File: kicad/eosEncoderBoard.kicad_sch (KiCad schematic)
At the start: 0 parts

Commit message: schematic half done
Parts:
- added DP1: Display1, Connector_PinSocket_2.54mm:PinSocket_1x04_P2.54mm_Vertical, symbol Connector_Generic:Conn_01x04
- added DP2: Display2, Connector_PinSocket_2.54mm:PinSocket_1x04_P2.54mm_Vertical, symbol Connector_Generic:Conn_01x04
- added DP3: Display3, Connector_PinSocket_2.54mm:PinSocket_1x04_P2.54mm_Vertical, symbol Connector_Generic:Conn_01x04
- added DP4: Display4, Connector_PinSocket_2.54mm:PinSocket_1x04_P2.54mm_Vertical, symbol Connector_Generic:Conn_01x04
- added R1, R10, R11, R12, R13, R14, R15, R16, R17, R18, R19, R2, R3, R4, R5, R6, R7, R8, R9: 10k, symbol Device:R_Small
- added SW1, SW2, SW3, SW4: RotaryEncoder, Rotary_Encoder:RotaryEncoder_Alps_EC11E-Switch_Vertical_H20mm_MountingHoles, symbol Device:RotaryEncoder_Switch_MP
- added U1: Teensy3.2, Teensy:Teensy30_31_32_LC, symbol Teensy:Teensy3.2
- added U2: PCA9548APW, Package_SO:TSSOP-24_4.4x7.8mm_P0.65mm, symbol Interface_Expansion:PCA9548APW
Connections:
- new net +3.3V: DP1.3 (Pin_3), DP2.3 (Pin_3), DP3.3 (Pin_3), DP4.3 (Pin_3), R1.1, R10.1, R11.1, R12.1, R13.2, R14.2, R15.2, R16.2, R17.2, R18.2, R19.2, R2.1, R3.1, R4.1, R5.1, R6.1, R7.1, R8.1, R9.1, U2.24 (VCC)
- new net A1: R2.2, SW1.A
- new net A2: R4.2, SW2.A
- new net A3: R7.2, SW3.A
- new net A4: R8.2, SW4.A
- new net B1: R1.2, SW1.B
- new net B2: R3.2, SW2.B
- new net B3: R5.2, SW3.B
- new net B4: R6.2, SW4.B
- new net GND: DP1.4 (Pin_4), DP2.4 (Pin_4), DP3.4 (Pin_4), DP4.4 (Pin_4), SW1.C, SW1.S2, SW2.C, SW2.S2, SW3.C, SW3.S2, SW4.C, SW4.S2, U2.1 (A0), U2.12 (GND), U2.2 (A1), U2.21 (A2)
- new net RST: R19.1, U2.3 (~{RESET})
- new net SCL: R17.1, U2.22 (SCL)
- new net SCL1: DP1.2 (Pin_2), R9.2, U2.5 (SC0)
- new net SCL2: DP2.2 (Pin_2), R11.2, U2.7 (SC1)
- new net SCL3: DP3.2 (Pin_2), R13.1, U2.9 (SC2)
- new net SCL4: DP4.2 (Pin_2), R15.1, U2.11 (SC3)
- new net SDA: R18.1, U2.23 (SDA)
- new net SDA1: DP1.1 (Pin_1), R10.2, U2.4 (SD0)
- new net SDA2: DP2.1 (Pin_1), R12.2, U2.6 (SD1)
- new net SDA3: DP3.1 (Pin_1), R14.1, U2.8 (SD2)
- new net SDA4: DP4.1 (Pin_1), R16.1, U2.10 (SD3)
- new net SW1: SW1.S1
- new net SW2: SW2.S1
- new net SW3: SW3.S1
- new net SW4: SW4.S1
- no-connect marks 0 -> 12
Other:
- note added: "Display Headers"
- note added: "Encoders"
- note added: "I2C Mux"

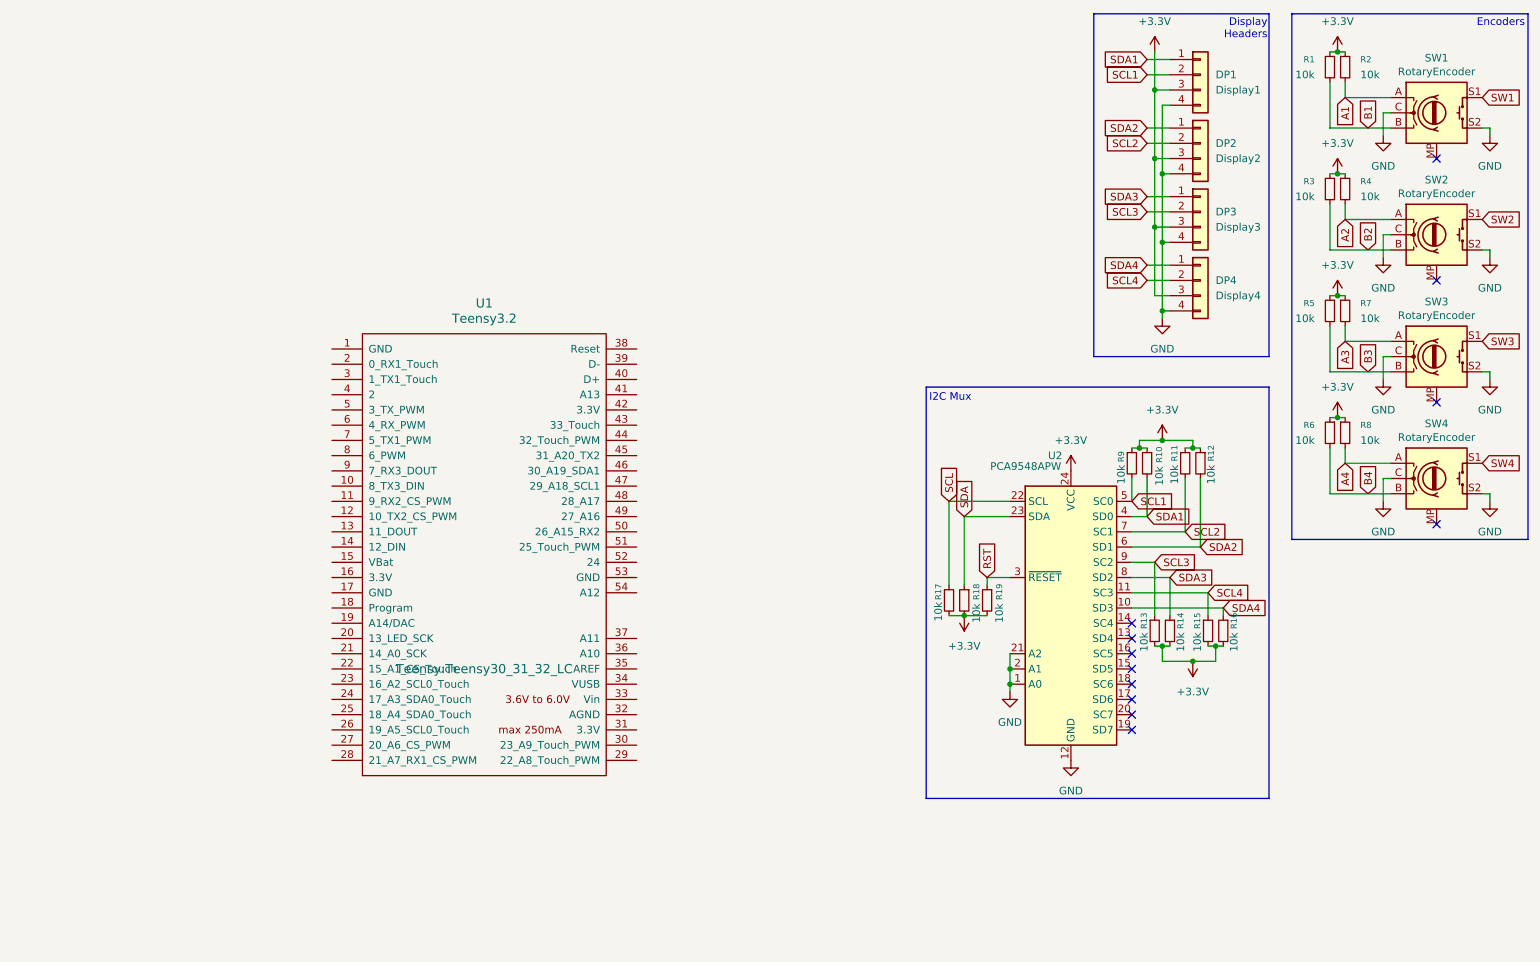
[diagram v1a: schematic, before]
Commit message: schematic basically done
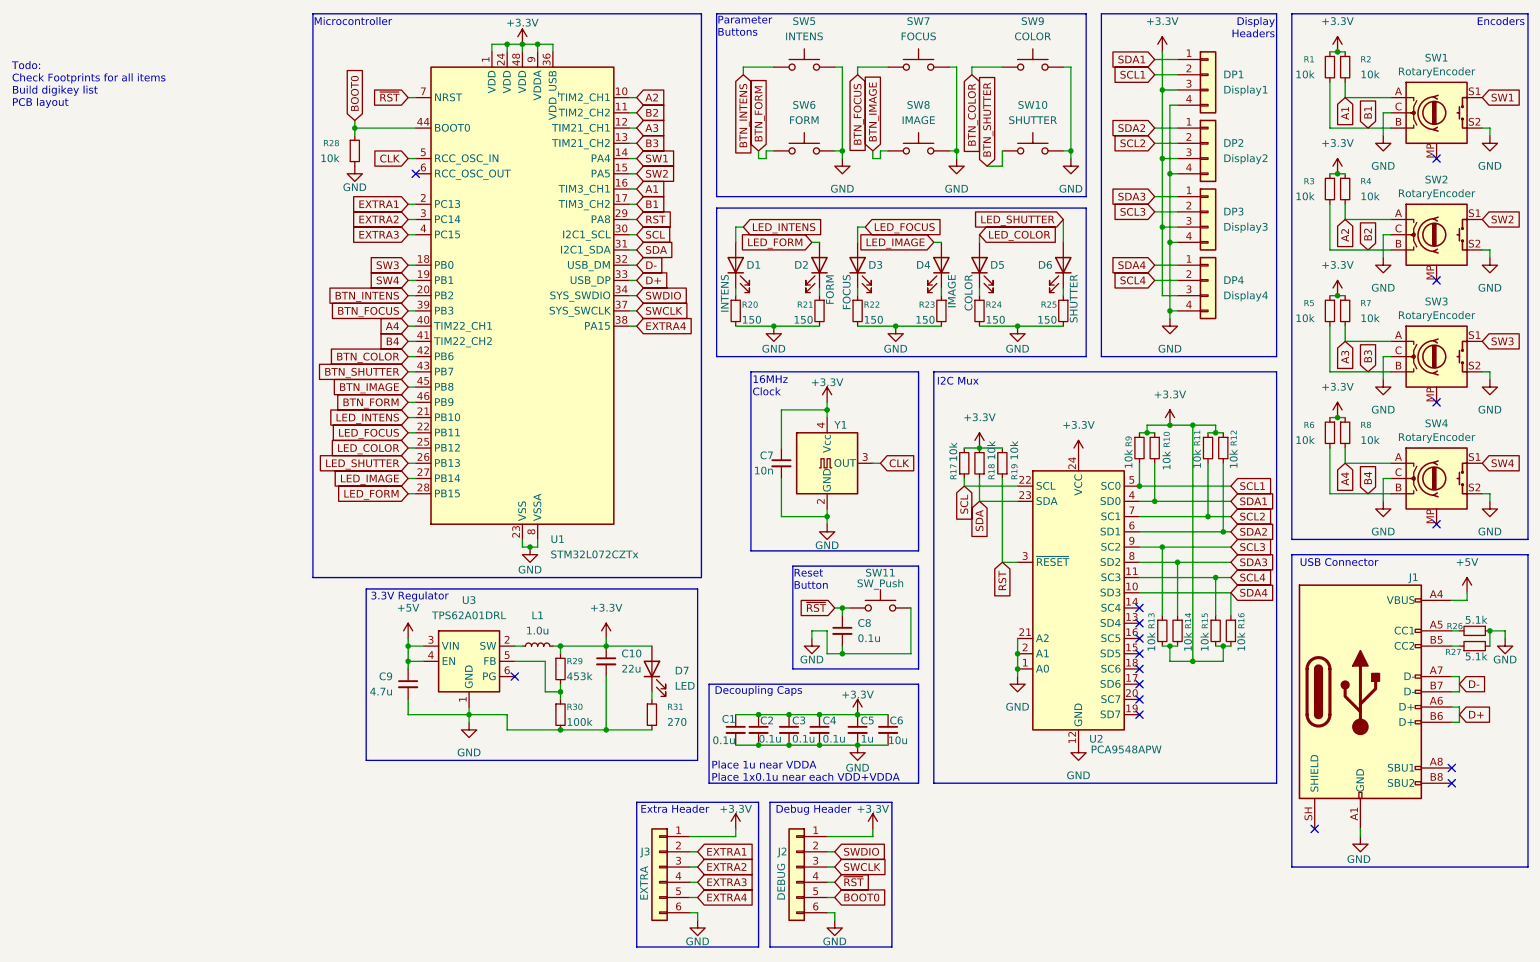
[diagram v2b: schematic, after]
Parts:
- removed U1: Teensy3.2, Teensy:Teensy30_31_32_LC, symbol Teensy:Teensy3.2
- added C1, C2, C3, C4, C8: 0.1u, symbol Device:C_Small
- added C10: 22u, symbol Device:C_Small
- added C5: 1u, symbol Device:C_Small
- added C6: 10u, symbol Device:C_Small
- added C7: 10n, symbol Device:C_Small
- added C9: 4.7u, symbol Device:C_Small
- added D1: INTENS, symbol Device:LED
- added D2: FORM, symbol Device:LED
- added D3: FOCUS, symbol Device:LED
- added D4: IMAGE, symbol Device:LED
- added D5: COLOR, symbol Device:LED
- added D6: SHUTTER, symbol Device:LED
- added D7: LED, symbol Device:LED
- added J1: USB_C_Receptacle_USB2.0_16P, Connector_USB:USB_C_Receptacle_GCT_USB4105-xx-A_16P_TopMnt_Horizontal, symbol Connector:USB_C_Receptacle_USB2.0_16P
- added J2: DEBUG, Connector_PinSocket_2.54mm:PinSocket_1x06_P2.54mm_Vertical, symbol Connector_Generic:Conn_01x06
- added J3: EXTRA, Connector_PinSocket_2.54mm:PinSocket_1x06_P2.54mm_Vertical, symbol Connector_Generic:Conn_01x06
- added L1: 1.0u, symbol Device:L_Small
- added R20, R21, R22, R23, R24, R25: 150, symbol Device:R_Small
- added R26, R27: 5.1k, symbol Device:R_Small
- added R28: 10k, symbol Device:R_Small
- added R29: 453k, symbol Device:R_Small
- added R30: 100k, symbol Device:R_Small
- added R31: 270, symbol Device:R_Small
- added SW10: SHUTTER, Button_Switch_Keyboard:SW_Cherry_MX_1.00u_PCB, symbol Switch:SW_Push
- added SW11: SW_Push, symbol Switch:SW_Push
- added SW5: INTENS, Button_Switch_Keyboard:SW_Cherry_MX_1.00u_PCB, symbol Switch:SW_Push
- added SW6: FORM, Button_Switch_Keyboard:SW_Cherry_MX_1.00u_PCB, symbol Switch:SW_Push
- added SW7: FOCUS, Button_Switch_Keyboard:SW_Cherry_MX_1.00u_PCB, symbol Switch:SW_Push
- added SW8: IMAGE, Button_Switch_Keyboard:SW_Cherry_MX_1.00u_PCB, symbol Switch:SW_Push
- added SW9: COLOR, Button_Switch_Keyboard:SW_Cherry_MX_1.00u_PCB, symbol Switch:SW_Push
- added U1: STM32L072CZTx, Package_QFP:LQFP-48_7x7mm_P0.5mm, symbol MCU_ST_STM32L0:STM32L072CZTx
- added U3: TPS62A01DRL, Package_TO_SOT_SMD:SOT-563, symbol Regulator_Switching:TPS62A01DRL
- added Y1: OSC16M-3.3I/S3T, Oscillator:Oscillator_SMD_Abracon_ASE-4Pin_3.2x2.5mm, symbol Oscillator:SG-8002CE
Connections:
- net +3.3V: now also C1.1, C10.1, C2.1, C3.1, C4.1, C5.1, C6.1, C7.1, D7.2 (A), J2.1 (Pin_1), J3.1 (Pin_1), L1.2, R29.1, U1.1 (VDD), U1.24 (VDD), U1.36 (VDD_USB), U1.48 (VDD), U1.9 (VDDA), Y1.4 (Vcc)
- net A1: now also U1.16 (PA6)
- net A2: now also U1.10 (PA0)
- net A3: now also U1.12 (PA2)
- net A4: now also U1.40 (PB4)
- net B1: now also U1.17 (PA7)
- net B2: now also U1.11 (PA1)
- net B3: now also U1.13 (PA3)
- net B4: now also U1.41 (PB5)
- net GND: now also C1.2, C10.2, C2.2, C3.2, C4.2, C5.2, C6.2, C7.2, C8.2, C9.2, J1.A1 (GND), J1.A12 (GND), J1.B1 (GND), J1.B12 (GND), J2.6 (Pin_6), J3.6 (Pin_6), R20.2, R21.2, R22.2, R23.2, R24.2, R25.2, R26.1, R27.2, R28.2, R30.2, R31.2, SW10.2, SW11.1, SW5.2, SW6.2, SW7.2, SW8.2, SW9.2, U1.23 (VSS), U1.35 (VSS), U1.47 (VSS), U1.8 (VSSA), U3.1 (GND), Y1.2 (GND)
- net RST: now also U1.29 (PA8)
- net SCL: now also U1.30 (PA9)
- net SDA: now also U1.31 (PA10)
- net SW1: now also U1.14 (PA4)
- net SW2: now also U1.15 (PA5)
- net SW3: now also U1.18 (PB0)
- net SW4: now also U1.19 (PB1)
- new net: D2.1 (K), R21.1
- new net: D7.1 (K), R31.1
- new net: L1.1, U3.2 (SW)
- new net: R29.2, R30.1, U3.5 (FB)
- new net: J1.A5 (CC1), R26.2
- new net: J1.B5 (CC2), R27.1
- new net: D3.1 (K), R22.1
- new net: D5.1 (K), R24.1
- new net: D6.1 (K), R25.1
- new net: D1.1 (K), R20.1
- new net: D4.1 (K), R23.1
- new net +5V: C9.1, J1.A4 (VBUS), J1.A9 (VBUS), J1.B4 (VBUS), J1.B9 (VBUS), U3.3 (VIN), U3.4 (EN)
- new net BOOT0: J2.5 (Pin_5), R28.1, U1.44 (BOOT0)
- new net BTN_COLOR: SW9.1, U1.42 (PB6)
- new net BTN_FOCUS: SW7.1, U1.39 (PB3)
- new net BTN_FORM: SW6.1, U1.46 (PB9)
- new net BTN_IMAGE: SW8.1, U1.45 (PB8)
- new net BTN_INTENS: SW5.1, U1.20 (PB2)
- new net BTN_SHUTTER: SW10.1, U1.43 (PB7)
- new net CLK: U1.5 (PH0), Y1.3 (OUT)
- new net D+: J1.A6 (D+), J1.B6 (D+), U1.33 (PA12)
- new net D-: J1.A7 (D-), J1.B7 (D-), U1.32 (PA11)
- new net EXTRA1: J3.2 (Pin_2), U1.2 (PC13)
- new net EXTRA2: J3.3 (Pin_3), U1.3 (PC14)
- new net EXTRA3: J3.4 (Pin_4), U1.4 (PC15)
- new net EXTRA4: J3.5 (Pin_5), U1.38 (PA15)
- new net LED_COLOR: D5.2 (A), U1.25 (PB12)
- new net LED_FOCUS: D3.2 (A), U1.22 (PB11)
- new net LED_FORM: D2.2 (A), U1.28 (PB15)
- new net LED_IMAGE: D4.2 (A), U1.27 (PB14)
- new net LED_INTENS: D1.2 (A), U1.21 (PB10)
- new net LED_SHUTTER: D6.2 (A), U1.26 (PB13)
- new net SWCLK: J2.3 (Pin_3), U1.37 (PA14)
- new net SWDIO: J2.2 (Pin_2), U1.34 (PA13)
- new net ~{RST}: C8.1, J2.4 (Pin_4), SW11.2, U1.7 (NRST)
- no-connect marks 12 -> 17
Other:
- note added: "16MHz Clock"
- note added: "3.3V Regulator"
- note added: "Debug Header"
- note added: "Decoupling Caps"
- note added: "Extra Header"
- note added: "Microcontroller"
- note added: "Parameter Buttons"
- note added: "Place 1u near VDDA Place 1x0.1u near each VDD+VDDA"
- note added: "Reset Button"
- note added: "Todo: Check Footprints for all items Build digikey list PCB layout"
- note added: "USB Connector"
- moved on the sheet: DP1, DP2, DP3, DP4, R10, R11, R12, R13, R14, R15, R16, R17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
